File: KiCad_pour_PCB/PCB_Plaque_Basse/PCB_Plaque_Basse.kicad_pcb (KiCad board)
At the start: 2 copper layers, 108 x 108 mm, 3 parts

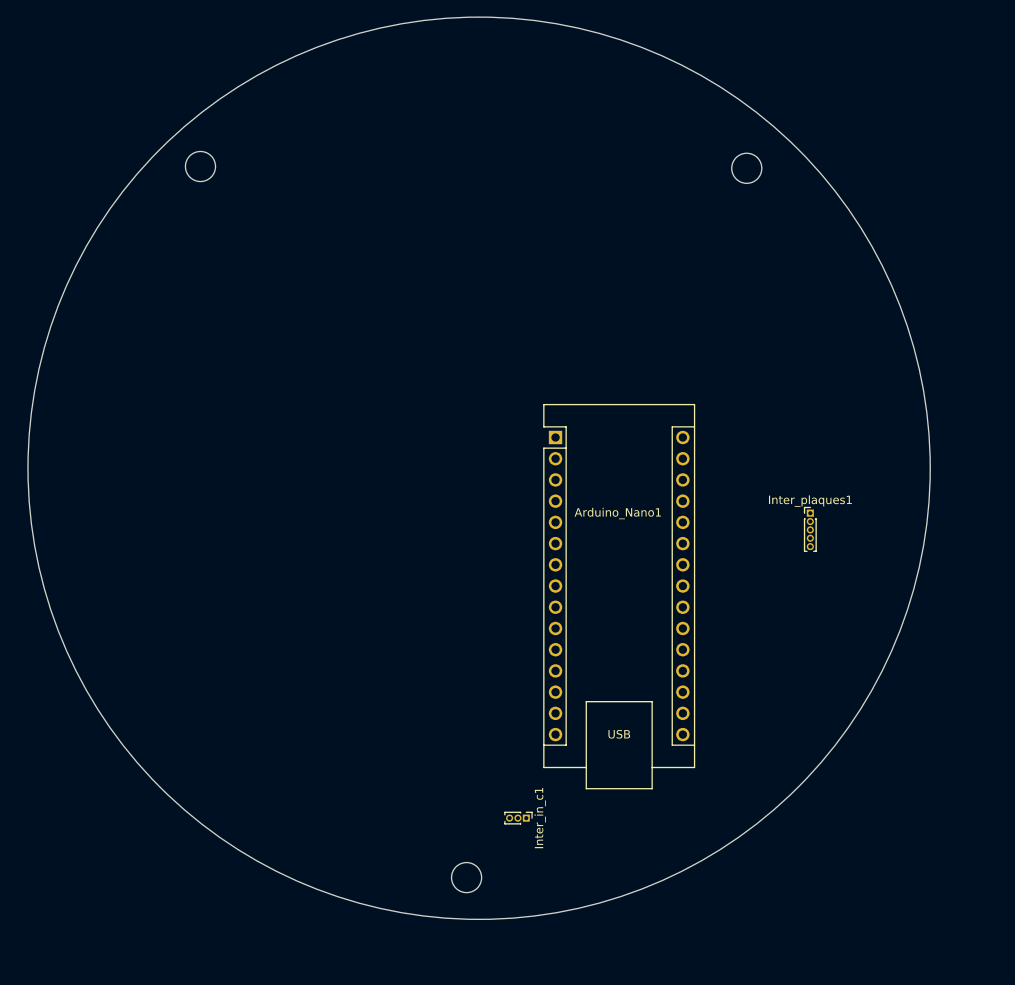
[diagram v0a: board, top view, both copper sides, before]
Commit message: PCB_Fin
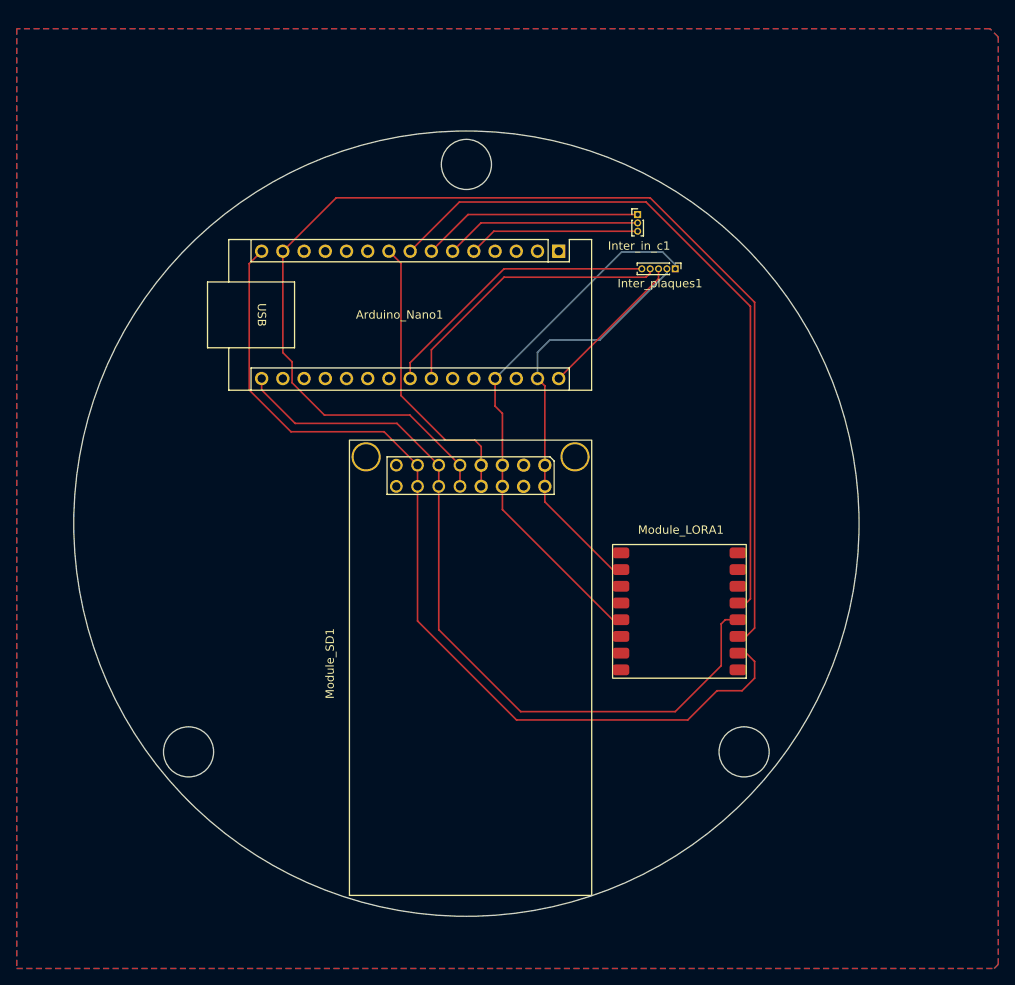
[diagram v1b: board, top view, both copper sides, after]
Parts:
- added Module_LORA1: ~, INSARIANNE_Lib:Module_LORA, F.Cu at (171.3, 99.8)
- added Module_SD1: ~, INSARIANNE_Lib:Module_SD, F.Cu at (152.8, 141.8)
- moved Inter_in_c1 73.5 mm to (158.3, 60.2), turned to 0 degrees
- moved Inter_plaques1 33.4 mm to (162.8, 66.8), turned to -90 degrees
- moved Arduino_Nano1 22.3 mm to (148.9, 64.6), turned to 180 degrees
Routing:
- net Net-(Arduino_Nano1-D11): track 0.00 -> 148.6 mm
- net Net-(Arduino_Nano1-D12): track 0.00 -> 111.5 mm
- net Net-(Arduino_Nano1-D13): track 0.00 -> 93.3 mm
- net Net-(Arduino_Nano1-D5): track 0.00 -> 85.1 mm
- net Net-(Arduino_Nano1-5V): track 0.00 -> 64.7 mm
- net Net-(Inter_plaques1-GND): track 0.00 -> 50.7 mm
- net Net-(Arduino_Nano1-D6): track 0.00 -> 34.8 mm
- net Net-(Arduino_Nano1-A4): track 0.00 -> 34.3 mm
- net Net-(Arduino_Nano1-A5): track 0.00 -> 33.9 mm
- net Net-(Arduino_Nano1-D4): track 0.00 -> 26.5 mm
- net Net-(Arduino_Nano1-D3): track 0.00 -> 23.6 mm
- net Net-(Arduino_Nano1-D2): track 0.00 -> 20.6 mm
- net Net-(Arduino_Nano1-Vin): track 0.00 -> 18.1 mm
- added copper zone on B.Cu, net Net-(Inter_plaques1-GND)
- added copper zone on F.Cu, net Net-(Inter_plaques1-GND)
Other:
- board size 108 x 108 mm -> 94 x 94 mm
